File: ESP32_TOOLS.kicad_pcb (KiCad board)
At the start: 2 copper layers, 11 parts, among them J1 LED, J3 OLED, SW1 UP_SW, SW2 DOWN_SW, SW3 OK_SW, SW4 LEFT_SW, SW5 RIGHT_SW

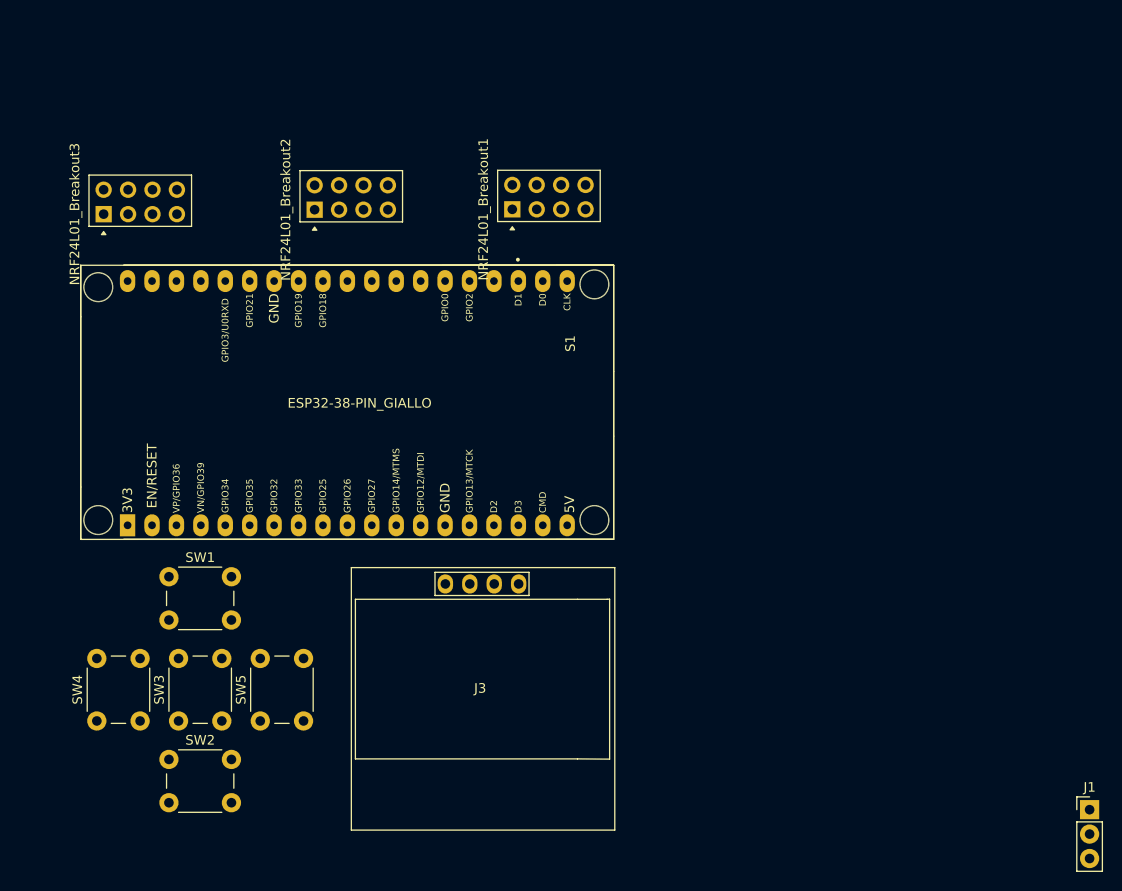
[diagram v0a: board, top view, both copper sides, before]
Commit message: fofo1
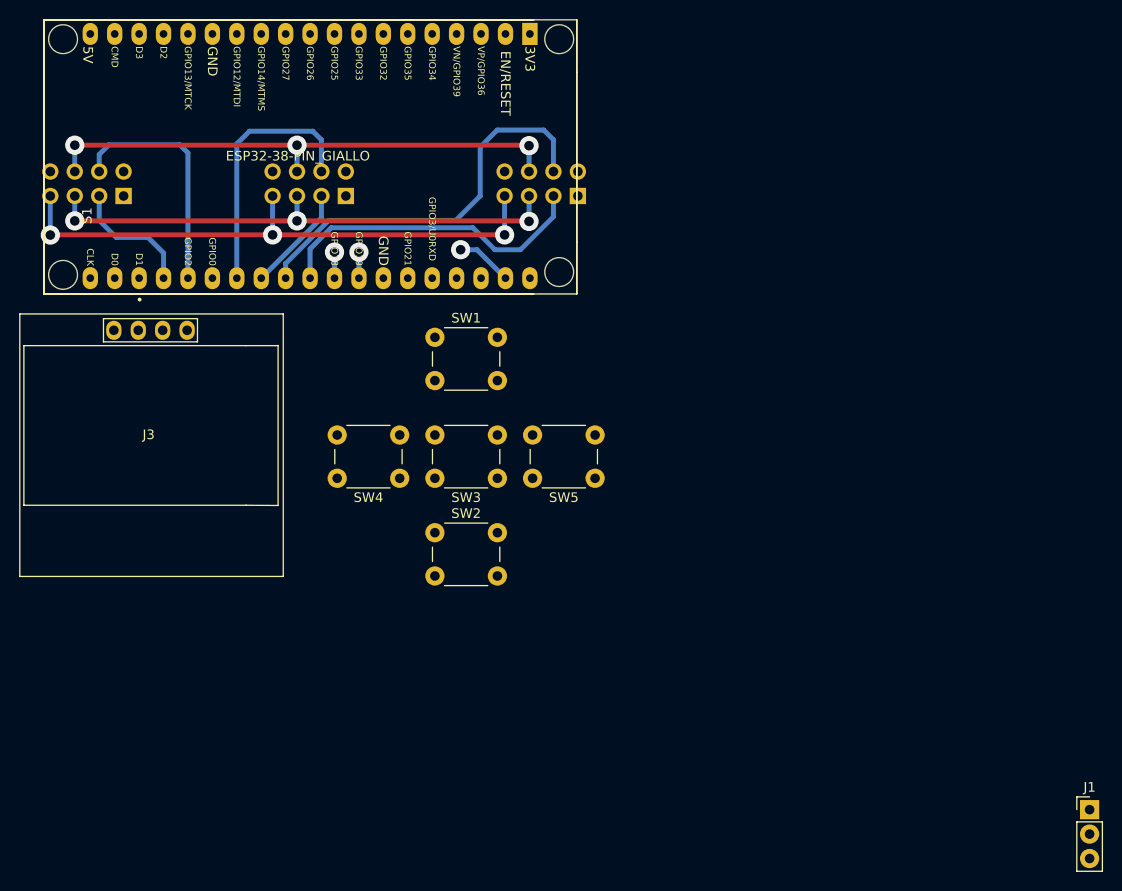
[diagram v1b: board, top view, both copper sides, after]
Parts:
- NRF24L01_Breakout1, NRF24L01_Breakout2, NRF24L01_Breakout3: moved to B.Cu
- moved S1 59.9 mm to (152.5, 67.6), turned to 90 degrees
- moved J3 43.4 mm to (163.6, 81.7)
- moved SW5 43.0 mm to (210.1, 86.5), turned to 180 degrees
- moved SW3 41.7 mm to (199.9, 86.5), turned to 180 degrees
- moved SW4 40.4 mm to (189.8, 86.5), turned to 180 degrees
- moved SW1 37.2 mm to (193.4, 71.8)
- moved SW2 36.3 mm to (193.4, 92.2)
- moved NRF24L01_Breakout1 6.96 mm to (208.3, 57.1)
- moved NRF24L01_Breakout2 3.55 mm to (184.2, 57.1)
- moved NRF24L01_Breakout3 2.81 mm to (161.0, 57.1)
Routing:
- net /MISO: track 0.00 -> 62.1 mm, vias 0 -> 4
- net /MOSI: track 0.00 -> 61.4 mm, vias 0 -> 4
- net /SCK: track 0.00 -> 57.7 mm, vias 0 -> 4
- net /SS_ALTO: track 0.00 -> 41.8 mm
- net /CE_ALTO: track 0.00 -> 33.8 mm
- net /SS_CENTRO: track 0.00 -> 27.0 mm
- net /SS_BASSO: track 0.00 -> 24.8 mm
- net /CE_BASSO: track 0.00 -> 13.3 mm
- net /CE_CENTRO: track 0.00 -> 11.1 mm
